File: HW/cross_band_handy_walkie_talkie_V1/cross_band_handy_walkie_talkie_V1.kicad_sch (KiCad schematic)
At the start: 29 parts

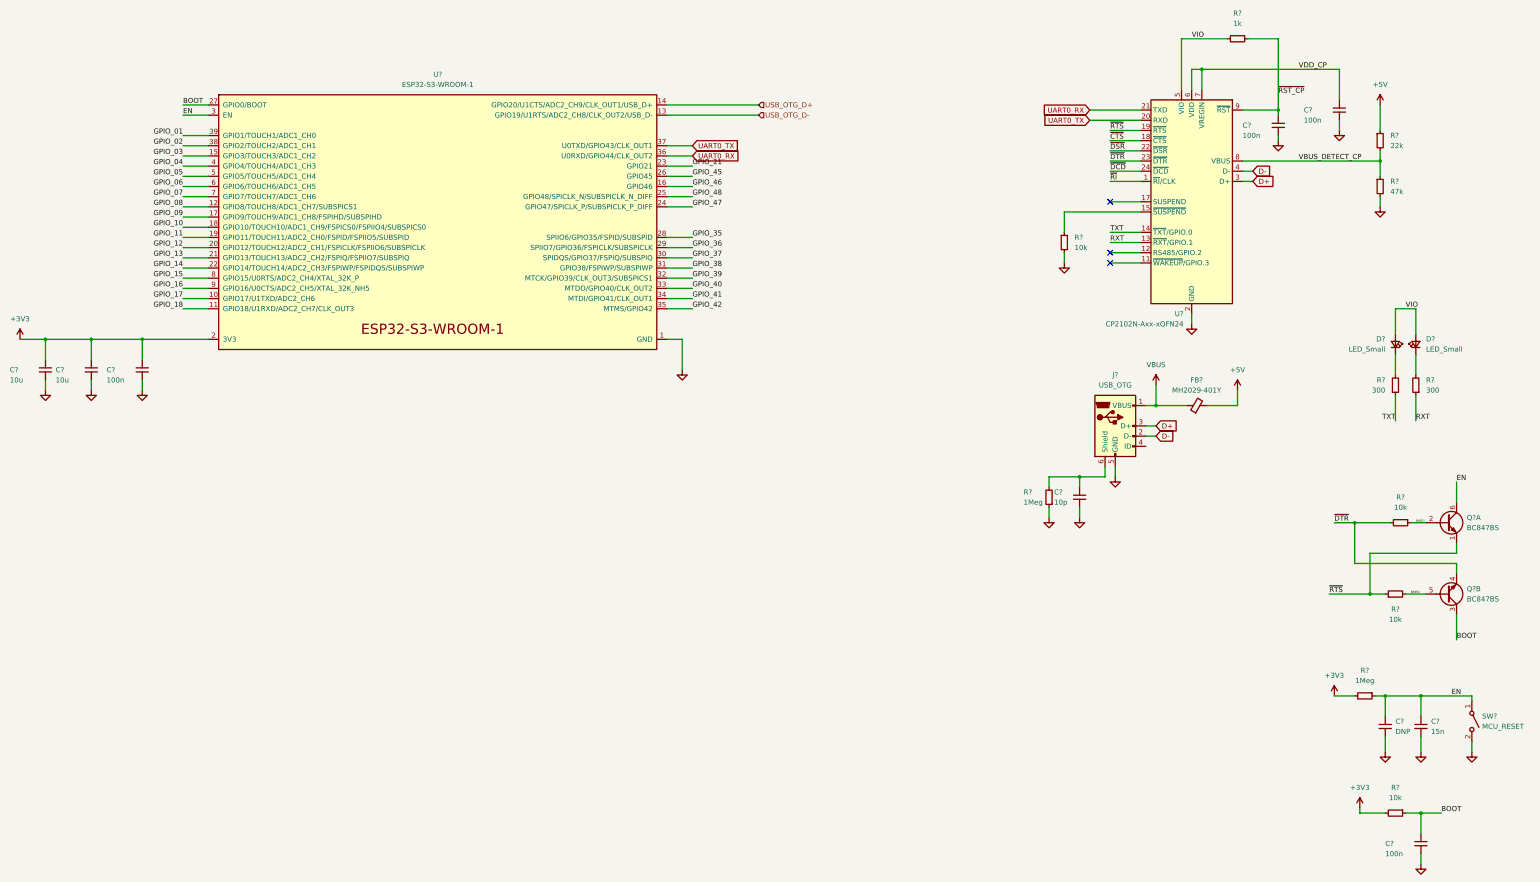
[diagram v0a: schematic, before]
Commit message: F
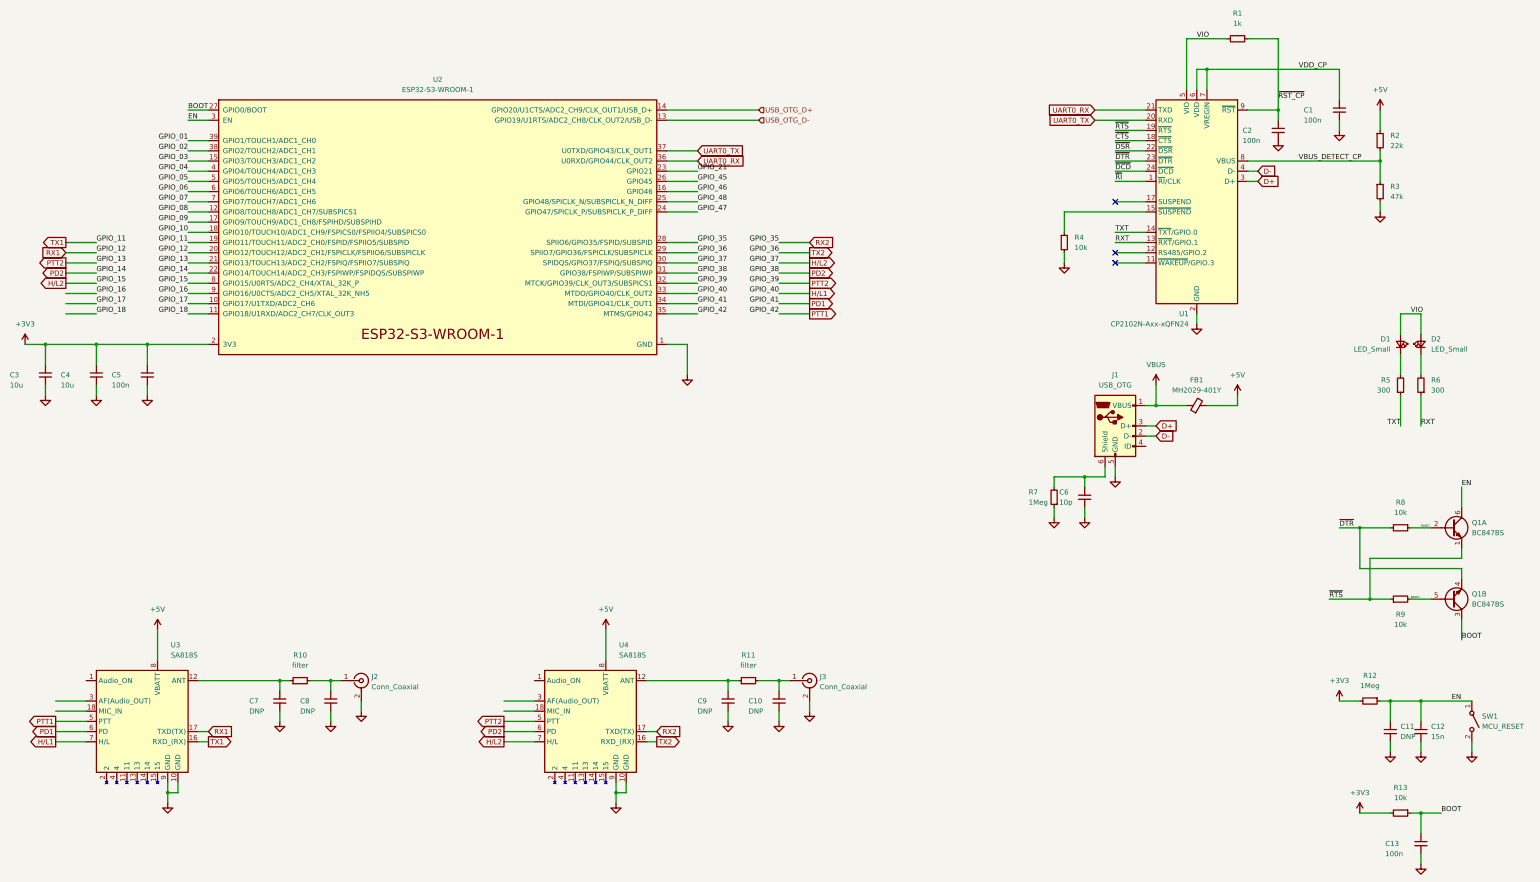
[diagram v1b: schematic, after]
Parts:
- added C10, C7, C8, C9: DNP, Capacitor_SMD:C_0603_1608Metric_Pad1.08x0.95mm_HandSolder, symbol Device:C_Small
- added J2, J3: Conn_Coaxial, Connector_Coaxial:SMA_Amphenol_901-144_Vertical, symbol Connector:Conn_Coaxial
- added R10, R11: filter, Resistor_SMD:R_1206_3216Metric_Pad1.30x1.75mm_HandSolder, symbol Device:R_Small
- added U3, U4: SA818S, Z_mycustom_footprint_lib:SA818S, symbol My_custom_lib:SA818S
- gave numbers to parts that had none: 28
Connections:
- net GPIO_37 is gone; now on net H/L2: U2.30 (SPIDQS/GPIO37/FSPIQ/SUBSPIQ)
- net GPIO_38 is gone; now on net PD2: U2.31 (GPIO38/FSPIWP/SUBSPIWP)
- net GPIO_39 is gone; now on net PTT2: U2.32 (MTCK/GPIO39/CLK_OUT3/SUBSPICS1)
- net +5V: now also U3.8 (VBATT), U4.8 (VBATT)
- net GND: now also C10.2, C7.2, C8.2, C9.2, J2.2 (Ext), J3.2 (Ext), U3.10 (GND), U3.9 (GND), U4.10 (GND), U4.9 (GND)
- net GPIO_11 renamed TX1
- net TX1: now also U3.16 (RXD_(RX))
- net GPIO_12 renamed RX1
- net RX1: now also U3.17 (TXD(TX))
- net GPIO_13 renamed PTT2
- net PTT2: now also U4.5 (PTT)
- net GPIO_14 renamed PD2
- net PD2: now also U4.6 (PD)
- net GPIO_15 renamed H/L2
- net H/L2: now also U4.7 (H/L)
- net GPIO_35 renamed RX2
- net RX2: now also U4.17 (TXD(TX))
- net GPIO_36 renamed TX2
- net TX2: now also U4.16 (RXD_(RX))
- net GPIO_40 renamed H/L1
- net H/L1: now also U3.7 (H/L)
- net GPIO_41 renamed PD1
- net PD1: now also U3.6 (PD)
- net GPIO_42 renamed PTT1
- net PTT1: now also U3.5 (PTT)
- new net: C9.1, R11.1, U4.12 (ANT)
- new net: C7.1, R10.1, U3.12 (ANT)
- new net: C8.1, J2.1 (In), R10.2
- new net: C10.1, J3.1 (In), R11.2
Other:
- moved on the sheet: C11, C12, C2, C3, C4, C5, C6, D1, D2, Q1A, Q1B, R12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

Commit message: h
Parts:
- added C14, C16, C18: 1u, Capacitor_SMD:C_0603_1608Metric_Pad1.08x0.95mm_HandSolder, symbol Device:C_Small
- added C15, C28, C29: 10u, Capacitor_SMD:C_0603_1608Metric_Pad1.08x0.95mm_HandSolder, symbol Device:C_Small
- added C17, C19, C22: 1uF, Capacitor_SMD:C_0805_2012Metric, symbol Device:C
- added C20: 1nF, Capacitor_SMD:C_0805_2012Metric, symbol Device:C
- added C21: 10uF, Capacitor_SMD:C_0805_2012Metric, symbol Device:C
- added C23: 1u-10u?, Capacitor_SMD:C_0603_1608Metric_Pad1.08x0.95mm_HandSolder, symbol Device:C_Small
- added C24: 47n, Capacitor_SMD:C_0603_1608Metric_Pad1.08x0.95mm_HandSolder, symbol Device:C_Small
- added C25: 47nF, Capacitor_SMD:C_0805_2012Metric, symbol Device:C
- added C26, C27: 4u7, Capacitor_SMD:C_0603_1608Metric_Pad1.08x0.95mm_HandSolder, symbol Device:C_Small
- added R14: 10, Resistor_SMD:R_0603_1608Metric_Pad0.98x0.95mm_HandSolder, symbol Device:R_Small
- added R15: 10R, Resistor_SMD:R_0805_2012Metric, symbol Device:R
- added RV1, RV2, RV3: 10k, Potentiometer_SMD:Potentiometer_Vishay_TS53YL_Vertical, symbol Device:R_POT
- added U5: LM386, symbol Amplifier_Audio:LM386
- added U6: LM386, Package_SO:SOIC-8_3.9x4.9mm_P1.27mm, symbol Amplifier_Audio:LM386
- added U7: LT1129-3.3_SO8, Package_SO:SOIC-8_3.9x4.9mm_P1.27mm, symbol Regulator_Linear:LT1129-3.3_SO8
- added U8: MAX9814, Package_DFN_QFN:DFN-14-1EP_3x3mm_P0.4mm_EP1.78x2.35mm, symbol Amplifier_Audio:MAX9814
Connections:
- net +3V3: now also C27.1, U7.1 (OUT), U7.2 (SENSE)
- net +5V: now also C15.1, C26.1, C28.2, C29.2, U5.6 (V+), U7.8 (IN)
- net GND: now also C14.2, C15.2, C20.2, C21.2, C24.2, C25.2, C26.2, C27.2, C28.1, C29.1, RV1.3, RV2.3, U5.2 (-), U5.4 (GND), U6.2 (-), U6.4 (GND), U7.3 (GND), U7.6 (GND), U7.7 (GND)
- net MIC_OUT: now reaches U3.18 (MIC_IN)
- net MIC_OUT: now also U4.18 (MIC_IN), C18.2
- new net: C22.1, U6.1 (GAIN)
- new net: C22.2, U6.8 (GAIN)
- new net: RV3.1, U5.1 (GAIN)
- new net: RV1.2, U5.3 (+)
- new net: C18.1, R14.2, U5.5
- new net: C14.1, U5.7 (BYPASS)
- new net: C23.1, U5.8 (GAIN)
- new net: C24.1, R14.1
- new net: C25.1, R15.2
- new net: U8.11 (GND), U8.15 (GND), U8.4 (GND), U8.7 (GND)
- new net: C20.1, RV2.2, U6.3 (+)
- new net: C21.1, U6.7 (BYPASS)
- new net: C16.2, RV1.1
- new net: C17.2, RV2.1
- new net: C19.1, R15.1, U6.5
- new net: C23.2, RV3.2
- new net AF_TRX: C17.1
- new net MIC_IN: C16.1
- new net SPKR: C19.2
- new net VCC: U6.6 (V+)
- no-connect marks 3 -> 4
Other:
- note added: "750mA max current"
- note added: "SPEAKER AMP"
- moved on the sheet: C1, C10, C2, C3, C4, C5, C6, C7, C8, C9, D1, D2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

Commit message: b
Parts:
- removed C10, C7, C8, C9: DNP, Capacitor_SMD:C_0603_1608Metric_Pad1.08x0.95mm_HandSolder, symbol Device:C_Small
- removed J2: Conn_Coaxial, Connector_Coaxial:SMA_Amphenol_901-144_Vertical, symbol Connector:Conn_Coaxial
- removed R10, R11: filter, Resistor_SMD:R_1206_3216Metric_Pad1.30x1.75mm_HandSolder, symbol Device:R_Small
- added C10: 2.2uF, Capacitor_SMD:C_0805_2012Metric, symbol Device:C
- added C30: 1uF, Capacitor_SMD:C_0805_2012Metric, symbol Device:C
- added C7, C8: 100nF, Capacitor_SMD:C_0805_2012Metric, symbol Device:C
- added C9: 470nF, Capacitor_SMD:C_0805_2012Metric, symbol Device:C
- added FL? (x2): LFCN-160, Filter:Filter_Mini-Circuits_FV1206, symbol RF_Filter:LFCN-160
- added J4, J5: Conn_01x03, Connector_PinHeader_2.54mm:PinHeader_1x03_P2.54mm_Vertical, symbol Connector_Generic:Conn_01x03
- added J6: Conn_01x03, Jumper:SolderJumper-3_P2.0mm_Open_TrianglePad1.0x1.5mm_NumberLabels, symbol Connector_Generic:Conn_01x03
- added J? (x6): pin, Connector_PinHeader_2.54mm:PinHeader_1x01_P2.54mm_Vertical, symbol Connector_Generic:Conn_01x01
- added J?: Conn_Coaxial, Connector_Coaxial:SMA_Amphenol_901-144_Vertical, symbol Connector:Conn_Coaxial
- added L1: Ferrit, Resistor_SMD:R_0805_2012Metric_Pad1.20x1.40mm_HandSolder, symbol Device:L
- added R16: #2.2k, Resistor_SMD:R_0805_2012Metric, symbol Device:R
- added R17: 150k, Resistor_SMD:R_0805_2012Metric, symbol Device:R
- added R18: 1k, Resistor_SMD:R_0805_2012Metric, symbol Device:R
- added R19: 100k, Resistor_SMD:R_0805_2012Metric, symbol Device:R
- added U? (x8): TS5A63157DBV, Package_TO_SOT_SMD:SOT-23-6, symbol Analog_Switch:TS5A63157DBV
- U8: LCSC (none) -> C41714
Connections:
- net +3V3: now also J4.3 (Pin_3), J5.3 (Pin_3), L1.1
- net AF_TRX: no longer C17.1
- net GND: now also U8.11 (GND), U8.13 (MICBIAS), U8.15 (GND), U8.4 (GND), U8.7 (GND), U8.8 (MICIN), C10.2, C30.1, C7.1, C8.1, C9.2, FL?.2 (GND), FL?.2 (GND), FL?.4 (GND), FL?.4 (GND), J4.1 (Pin_1), J5.1 (Pin_1), J?.2 (Ext), R16.1, R17.1, R19.2
- net MIC_IN: now also J?.1 (Pin_1), U?.4, U?.4; no longer C16.1
- net at U4.12 (ANT): now also FL?.1 (IN)
- net at U3.12 (ANT): now also FL?.1 (IN)
- net at U3.3 (AF(Audio_OUT)): now also U?.3
- net at U4.3 (AF(Audio_OUT)): now also U?.1
- net at J3.1 (In): now also FL?.3 (OUT)
- net at U8.1 (CT): now also C7.2
- net at U8.10 (GAIN): now also R18.1
- net at U8.12 (BIAS): now also C9.1
- net at U8.14 (TH): now also R17.2, R19.1
- net -SLEEP: now reaches U8.2 (~{SHDN})
- net at U8.3 (CG): now also C10.1
- net at U8.5 (VDD): now also C30.2, L1.2
- net at U8.6 (MICOUT): now also J6.1 (Pin_1), J?.1 (Pin_1), U?.3
- net MIC_AR: now reaches U8.9 (A/R)
- net MIC_AR: now also J5.2 (Pin_2)
- removed net MIC_OUT: C18.2, U3.18 (MIC_IN), U4.18 (MIC_IN)
- new net: U3.18 (MIC_IN), U?.1
- new net: U4.18 (MIC_IN), U?.3
- new net: FL?.3 (OUT), J?.1 (In)
- new net AUDIO_IN: C16.1, J?.1 (Pin_1), U?.4
- new net AUDIO_OUT: C18.2, J?.1 (Pin_1), U?.3, U?.4
- new net MIC-AMP_IN: C8.2, R16.2
- new net MIC-DIGI_IN: J6.3 (Pin_3)
- new net MIC_GAIN: J4.2 (Pin_2), R18.2
- new net TRX_MIC: J6.2 (Pin_2)
- new net esp audio: J?.1 (Pin_1), J?.1 (Pin_1), U?.1, U?.1
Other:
- note added: "???"
- note added: "MIC AMP"
- note added: "VDD: 1:2000 NC: 1:4000 GND: 1:500"
- note added: "VDD: 40dB NC: 60dB GND: 50dB"
- moved on the sheet: C1, C11, C12, C13, C14, C15, C16, C17, C18, C19, C20, C21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
